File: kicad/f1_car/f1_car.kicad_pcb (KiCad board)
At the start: 2 copper layers, 26.1 x 55.9 mm, 2 parts, among them J4 Conn_01x12_Pin, U1 ESP32-C3-DevKitC-02

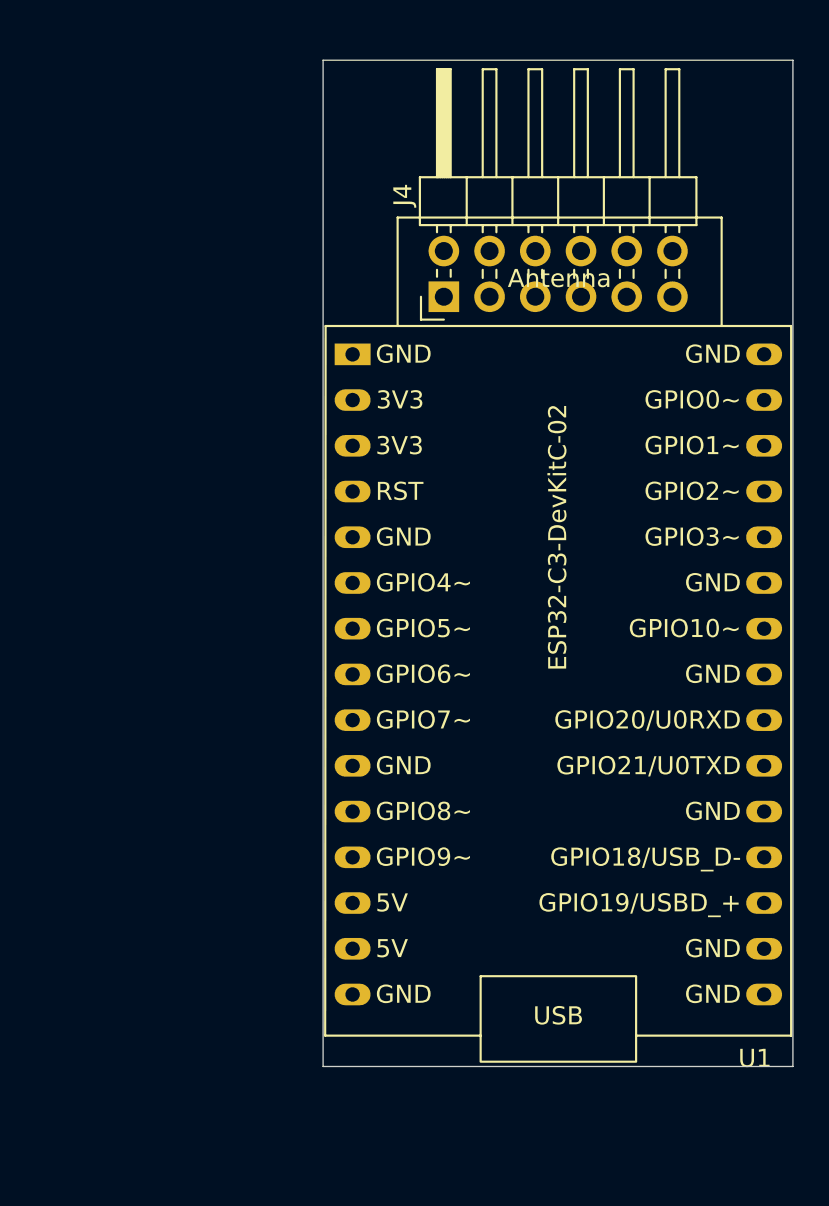
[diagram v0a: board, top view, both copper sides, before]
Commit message: first finished pcb
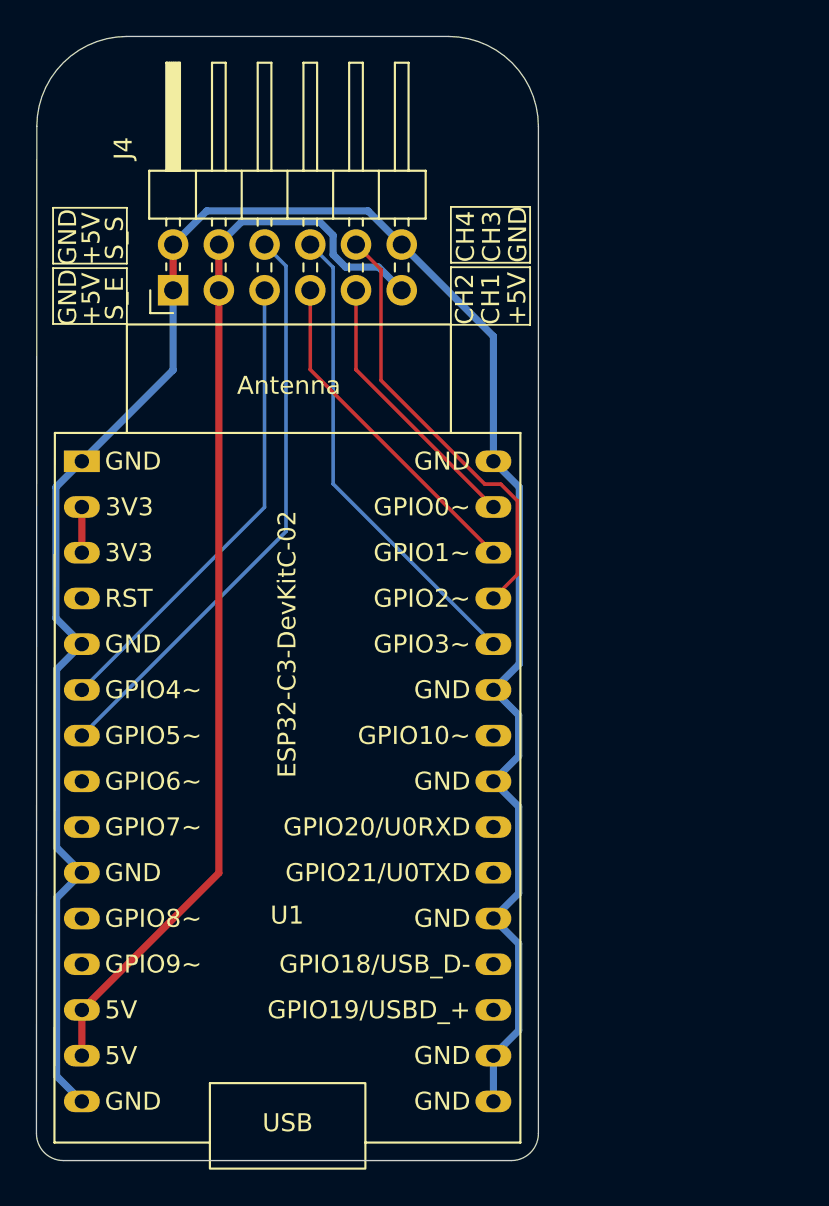
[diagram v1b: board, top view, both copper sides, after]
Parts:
- moved U1 16.2 mm to (134.3, 91.0)
- moved J4 15.0 mm to (139.4, 81.5)
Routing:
- net GND: track 0.00 -> 121.9 mm
- net +5V: track 0.00 -> 61.1 mm
- net SERVO_SIGNAL: track 0.00 -> 32.5 mm
- net CH4: track 0.00 -> 26.4 mm
- net ESC_SIGNAL: track 0.00 -> 26.4 mm
- net CH3: track 0.00 -> 24.4 mm
- net CH2: track 0.00 -> 18.8 mm
- net CH1: track 0.00 -> 15.2 mm
- net +3V3: track 0.00 -> 2.54 mm
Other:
- board size 26.1 x 55.9 mm -> 27.9 x 62.4 mm
- board text added: "+5V"
- board text added: "CH1"
- board text added: "CH2"
- board text added: "CH3"
- board text added: "CH4"
- board text added: "GND"
- board text added: "S_E"
- board text added: "S_S"
